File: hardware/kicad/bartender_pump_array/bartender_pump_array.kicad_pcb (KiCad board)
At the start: 2 copper layers, 56 x 61.8 mm, 43 parts, among them J1 Pump 1, J10 Pump 10, J11 12V INPUT, J12 Conn_01x12_Female, J2 Pump 2, J3 Pump 3, J4 Pump 4, J5 Pump 5, J6 Pump 6, J7 Pump 7, J8 Pump 8, J9 Pump 9, Q1 TIP120, Q10 TIP120, Q2 TIP120, Q3 TIP120, Q4 TIP120, Q5 TIP120, Q6 TIP120, Q7 TIP120, Q8 TIP120, Q9 TIP120

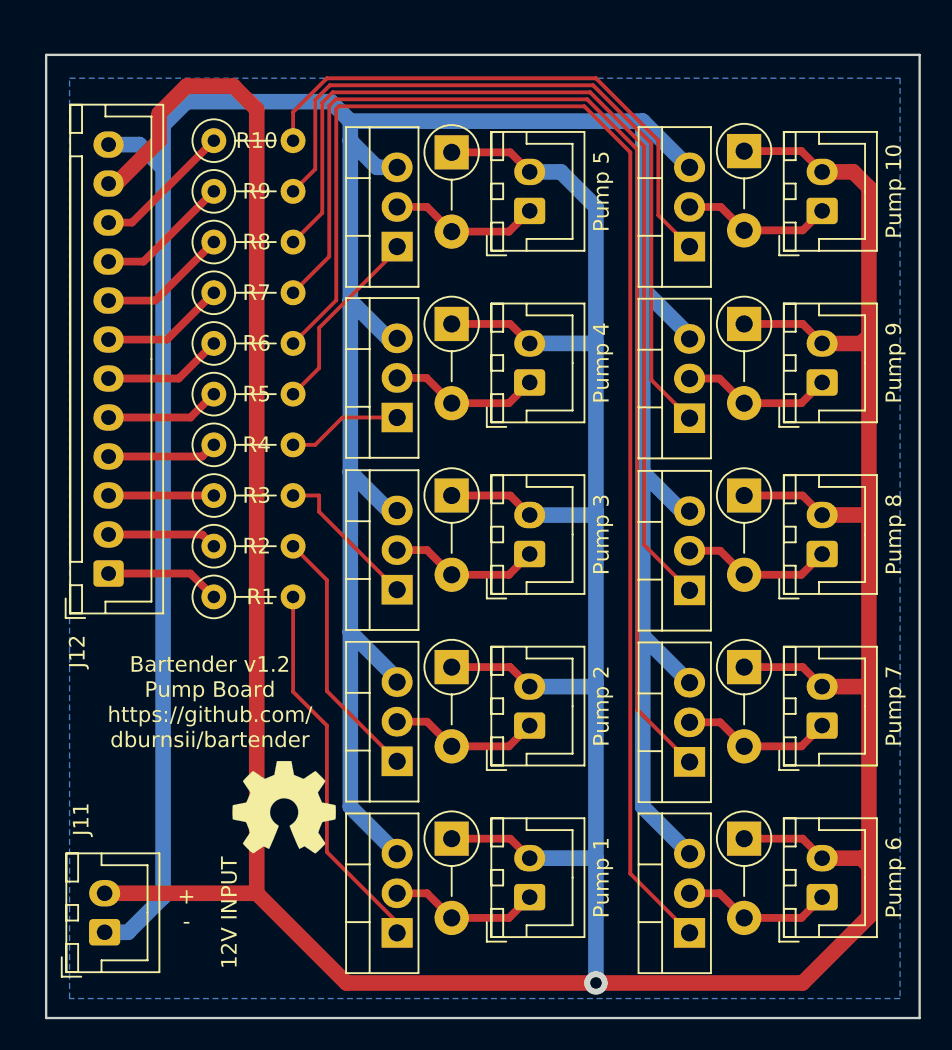
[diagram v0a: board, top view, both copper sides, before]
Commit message: Got wifi up and running, started work on the Mini
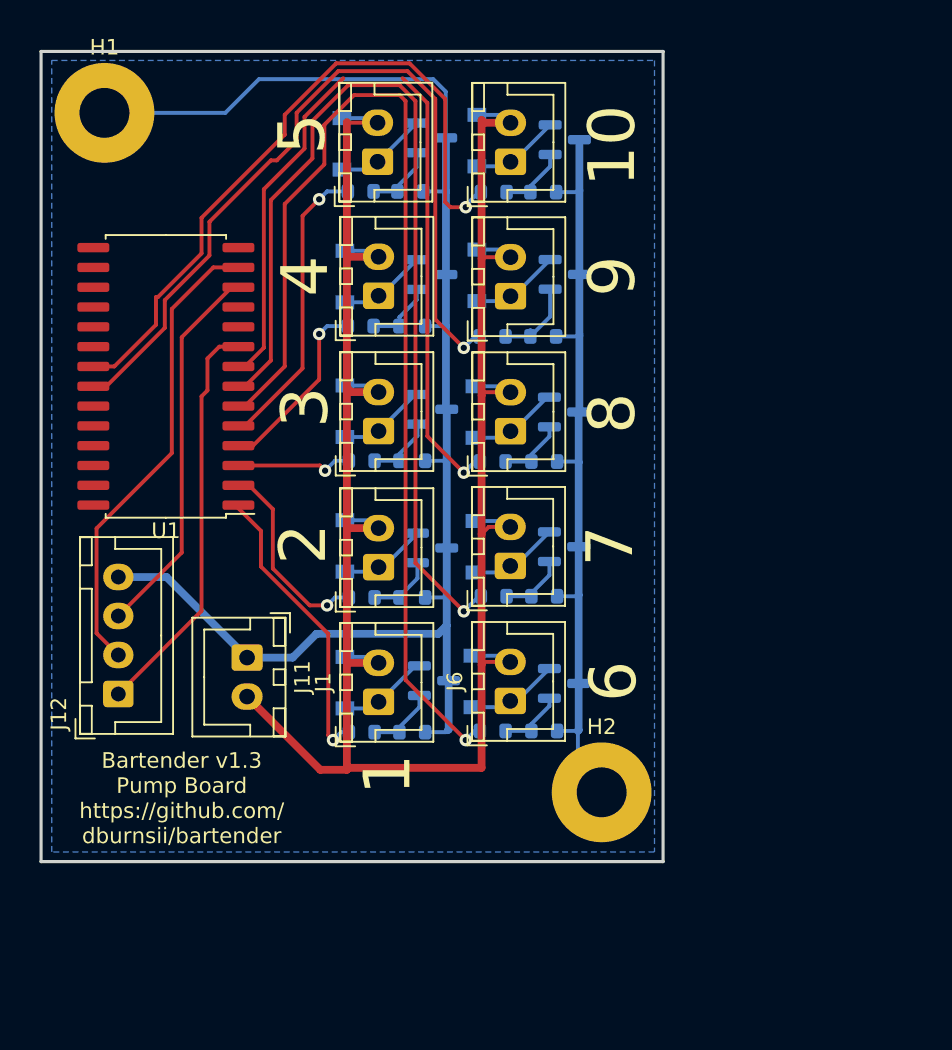
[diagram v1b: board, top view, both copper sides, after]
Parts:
- removed REF**: OSHW-Symbol_6.7x6mm_SilkScreen, Symbol:OSHW-Symbol_6.7x6mm_SilkScreen
- added H1: MountingHole_Pad, MountingHole:MountingHole_3.2mm_M3_Pad, F.Cu at (31.0, 45.5)
- added H2: MountingHole_Pad, MountingHole:MountingHole_3.2mm_M3_Pad, F.Cu at (62.9, 89.0)
- added R11: R_Small_US, Resistor_SMD:R_0603_1608Metric, B.Cu at (50.7, 85.2)
- added R12: R_Small_US, Resistor_SMD:R_0603_1608Metric, B.Cu at (50.7, 76.5)
- added R13: R_Small_US, Resistor_SMD:R_0603_1608Metric, B.Cu at (50.7, 67.8)
- added R14: R_Small_US, Resistor_SMD:R_0603_1608Metric, B.Cu at (50.7, 59.1)
- added R15: R_Small_US, Resistor_SMD:R_0603_1608Metric, B.Cu at (50.6, 50.5)
- added R16: R_Small_US, Resistor_SMD:R_0603_1608Metric, B.Cu at (59.2, 85.1)
- added R17: R_Small_US, Resistor_SMD:R_0603_1608Metric, B.Cu at (59.2, 76.5)
- added R18: R_Small_US, Resistor_SMD:R_0603_1608Metric, B.Cu at (59.2, 67.8)
- added R19: R_Small_US, Resistor_SMD:R_0603_1608Metric, B.Cu at (59.1, 59.8)
- added R20: R_Small_US, Resistor_SMD:R_0603_1608Metric, B.Cu at (59.1, 50.5)
- added U1: MCP23017_SO, Package_SO:SOIC-28W_7.5x17.9mm_P1.27mm, F.Cu at (34.9, 62.4)
- D1, D10, D2, D3, D4, D5, D6, D7, D8, D9: value DIODE -> 1N4148W; footprint Diode_THT:D_DO-41_SOD81_P5.08mm_Vertical_AnodeUp -> Diode_SMD:D_SOD-123; moved to B.Cu
- J1: value Pump 1 -> 1
- J10: value Pump 10 -> 10
- J11: value 12V INPUT -> 12V
- J12: value Conn_01x12_Female -> Conn_01x04_Female; footprint Connector_JST:JST_XH_B12B-XH-A_1x12_P2.50mm_Vertical -> Connector_JST:JST_XH_B4B-XH-A_1x04_P2.50mm_Vertical
- J2: value Pump 2 -> 2
- J3: value Pump 3 -> 3
- J4: value Pump 4 -> 4
- J5: value Pump 5 -> 5
- J6: value Pump 6 -> 6
- J7: value Pump 7 -> 7
- J8: value Pump 8 -> 8
- J9: value Pump 9 -> 9
- Q1, Q10, Q2, Q3, Q4, Q5, Q6, Q7, Q8, Q9: value TIP120 -> AO3400A; footprint Package_TO_SOT_THT:TO-220-3_Vertical -> Package_TO_SOT_SMD:SOT-23; moved to B.Cu
- R1, R10, R2, R3, R4, R5, R6, R7, R8, R9: footprint Resistor_THT:R_Axial_DIN0207_L6.3mm_D2.5mm_P5.08mm_Vertical -> Resistor_SMD:R_0603_1608Metric; moved to B.Cu
- moved R6 30.6 mm to (55.9, 85.1)
- moved R7 26.5 mm to (55.9, 76.5)
- moved J6 23.6 mm to (57.0, 83.2)
- moved R8 22.8 mm to (55.9, 67.8)
- moved J7 22.5 mm to (57.0, 74.5)
- moved J8 21.5 mm to (57.0, 65.9)
- moved J9 20.7 mm to (57.0, 57.2)
- moved J10 20.2 mm to (57.0, 48.6)
- moved R9 20.2 mm to (55.9, 59.8)
- moved D6 20.1 mm to (54.6, 81.9)
- moved J11 19.8 mm to (40.1, 80.4), turned to -90 degrees
- moved D7 18.9 mm to (54.7, 73.3)
- moved R10 18.2 mm to (55.9, 50.5)
- moved D8 18.1 mm to (54.7, 64.6)
- moved Q6 17.9 mm to (60.5, 82.0), turned to 0 degrees
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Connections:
- J12 pad 1: /P1 -> Net-(J12-Pad1)
- J12 pad 2: /P2 -> Net-(J12-Pad2)
- J12 pad 3: /P3 -> Net-(J12-Pad3)
- J12 pad 4: /P4 -> GND
- R1 pad 1: /P1 -> Net-(R1-Pad1)
- R10 pad 1: /P10 -> Net-(R10-Pad1)
- R2 pad 1: /P2 -> Net-(R2-Pad1)
- R3 pad 1: /P3 -> Net-(R3-Pad1)
- R4 pad 1: /P4 -> Net-(R4-Pad1)
- R5 pad 1: /P5 -> Net-(R5-Pad1)
- R6 pad 1: /P6 -> Net-(R6-Pad1)
- R7 pad 1: /P7 -> Net-(R7-Pad1)
- R8 pad 1: /P8 -> Net-(R8-Pad1)
- R9 pad 1: /P9 -> Net-(R9-Pad1)
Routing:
- net /12v: track 306.7 -> 144.7 mm, vias 1 -> 0
- net Net-(R6-Pad2): track 88.0 -> 4.23 mm
- net GND: track 219.7 -> 145.1 mm
- net Net-(R7-Pad2): track 74.9 -> 4.29 mm
- net Net-(R6-Pad1): track 0.00 -> 70.4 mm, vias 0 -> 1
- net Net-(R7-Pad1): track 0.00 -> 62.7 mm, vias 0 -> 1
- net Net-(R8-Pad2): track 61.7 -> 4.36 mm
- net Net-(R9-Pad1): track 0.00 -> 52.4 mm, vias 0 -> 1
- net Net-(R8-Pad1): track 0.00 -> 49.8 mm, vias 0 -> 1
- net Net-(R10-Pad1): track 0.00 -> 44.2 mm, vias 0 -> 1
- net Net-(Q9-Pad1): track 48.6 -> 5.56 mm
- net Net-(Q10-Pad1): track 35.4 -> 4.46 mm
- net Net-(J12-Pad2): track 0.00 -> 30.1 mm
- net Net-(J12-Pad1): track 0.00 -> 26.2 mm
- net Net-(J12-Pad3): track 0.00 -> 24.5 mm
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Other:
- board size 56 x 61.8 mm -> 39.9 x 51.9 mm
- net class Default removed
- board text added: "Bartender v1.3 Pump Board https://github.com/ dburnsii/bartender"
- board text removed: "+ -"
- board text removed: "Bartender v1.2 Pump Board https://github.com/ dburnsii/bartender"

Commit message: Updates for build, scale setup, new copy of pump board, etc
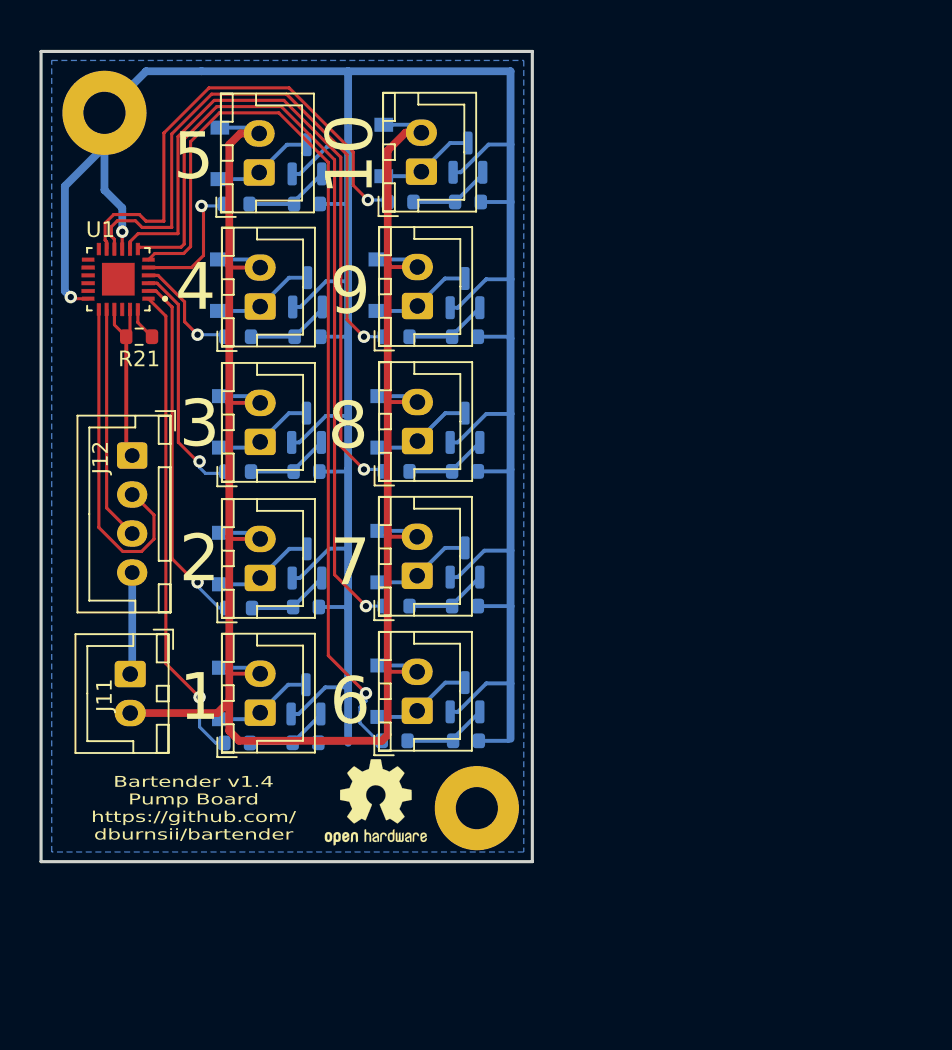
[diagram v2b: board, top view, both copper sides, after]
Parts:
- added R21: 1KR, Resistor_SMD:R_0603_1608Metric, F.Cu at (33.2, 59.8)
- added REF**: OSHW-Logo2_7.3x6mm_SilkScreen, Symbol:OSHW-Logo2_7.3x6mm_SilkScreen, F.Cu at (48.4, 89.7)
- H1, H2: footprint MountingHole:MountingHole_3.2mm_M3_Pad -> MountingHole:MountingHole_2.7mm_M2.5_Pad
- U1: value MCP23017_SO -> PCAL6416AHF,128; footprint Package_SO:SOIC-28W_7.5x17.9mm_P1.27mm -> PCAL6416AHF:QFN50P400X400X80-25N
- moved J12 15.3 mm to (32.8, 67.4), turned to -90 degrees
- moved Q1 8.30 mm to (43.9, 83.1), turned to 90 degrees
- moved Q3 8.14 mm to (43.9, 65.7), turned to 90 degrees
- moved Q2 8.08 mm to (44.0, 74.4), turned to 90 degrees
- moved Q5 8.07 mm to (44.0, 48.4), turned to 90 degrees
- moved D4 8.07 mm to (38.4, 56.5)
- moved H2 8.07 mm to (54.9, 90.0)
- moved R1 8.02 mm to (39.5, 85.9)
- moved Q4 8.02 mm to (44.0, 57.0), turned to 90 degrees
- moved R5 8.00 mm to (39.5, 51.3)
- moved D2 7.96 mm to (38.5, 74.0)
- moved D1 7.95 mm to (38.5, 82.7)
- moved R3 7.95 mm to (39.6, 68.5)
- moved D3 7.95 mm to (38.5, 65.3)
- moved R2 7.89 mm to (39.6, 77.2)
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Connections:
- D1 pad 2: Net-(J1-Pad1) -> Net-(D1-Pad2)
- D10 pad 2: Net-(J10-Pad1) -> Net-(D10-Pad2)
- D2 pad 2: Net-(J2-Pad1) -> Net-(D2-Pad2)
- D3 pad 2: Net-(J3-Pad1) -> Net-(D3-Pad2)
- D4 pad 2: Net-(J4-Pad1) -> Net-(D4-Pad2)
- D5 pad 2: Net-(J5-Pad1) -> Net-(D5-Pad2)
- D6 pad 2: Net-(J6-Pad1) -> Net-(D6-Pad2)
- D7 pad 2: Net-(J7-Pad1) -> Net-(D7-Pad2)
- D8 pad 2: Net-(J8-Pad1) -> Net-(D8-Pad2)
- D9 pad 2: Net-(J9-Pad1) -> Net-(D9-Pad2)
- J1 pad 1: Net-(J1-Pad1) -> Net-(D1-Pad2)
- J10 pad 1: Net-(J10-Pad1) -> Net-(D10-Pad2)
- J12 pad 1: Net-(J12-Pad1) -> +3V3
- J2 pad 1: Net-(J2-Pad1) -> Net-(D2-Pad2)
- J3 pad 1: Net-(J3-Pad1) -> Net-(D3-Pad2)
- J4 pad 1: Net-(J4-Pad1) -> Net-(D4-Pad2)
- J5 pad 1: Net-(J5-Pad1) -> Net-(D5-Pad2)
- J6 pad 1: Net-(J6-Pad1) -> Net-(D6-Pad2)
- J7 pad 1: Net-(J7-Pad1) -> Net-(D7-Pad2)
- J8 pad 1: Net-(J8-Pad1) -> Net-(D8-Pad2)
- J9 pad 1: Net-(J9-Pad1) -> Net-(D9-Pad2)
- Q1 pad 1: Net-(R1-Pad2) -> Net-(Q1-Pad1)
- Q1 pad 2: Net-(J1-Pad1) -> GND
- Q1 pad 3: GND -> Net-(D1-Pad2)
- Q10 pad 2: Net-(J10-Pad1) -> GND
- Q10 pad 3: GND -> Net-(D10-Pad2)
- Q2 pad 1: Net-(R2-Pad2) -> Net-(Q2-Pad1)
- Q2 pad 2: Net-(J2-Pad1) -> GND
- Q2 pad 3: GND -> Net-(D2-Pad2)
- Q3 pad 1: Net-(R3-Pad2) -> Net-(Q3-Pad1)
- Q3 pad 2: Net-(J3-Pad1) -> GND
- Q3 pad 3: GND -> Net-(D3-Pad2)
- Q4 pad 1: Net-(R4-Pad2) -> Net-(Q4-Pad1)
- Q4 pad 2: Net-(J4-Pad1) -> GND
- Q4 pad 3: GND -> Net-(D4-Pad2)
- Q5 pad 1: Net-(R5-Pad2) -> Net-(Q5-Pad1)
- Q5 pad 2: Net-(J5-Pad1) -> GND
- Q5 pad 3: GND -> Net-(D5-Pad2)
- Q6 pad 1: Net-(R6-Pad2) -> Net-(Q6-Pad1)
- Q6 pad 2: Net-(J6-Pad1) -> GND
- Q6 pad 3: GND -> Net-(D6-Pad2)
- Q7 pad 1: Net-(R7-Pad2) -> Net-(Q7-Pad1)
- Q7 pad 2: Net-(J7-Pad1) -> GND
- Q7 pad 3: GND -> Net-(D7-Pad2)
- Q8 pad 1: Net-(R8-Pad2) -> Net-(Q8-Pad1)
- Q8 pad 2: Net-(J8-Pad1) -> GND
- Q8 pad 3: GND -> Net-(D8-Pad2)
- Q9 pad 2: Net-(J9-Pad1) -> GND
- Q9 pad 3: GND -> Net-(D9-Pad2)
- R1 pad 2: Net-(R1-Pad2) -> Net-(Q1-Pad1)
- R11 pad 1: GND -> Net-(Q1-Pad1)
- R11 pad 2: Net-(R1-Pad2) -> GND
- R12 pad 1: GND -> Net-(Q2-Pad1)
- R12 pad 2: Net-(R2-Pad2) -> GND
- R13 pad 1: GND -> Net-(Q3-Pad1)
- R13 pad 2: Net-(R3-Pad2) -> GND
- R14 pad 1: GND -> Net-(Q4-Pad1)
- R14 pad 2: Net-(R4-Pad2) -> GND
- R15 pad 1: GND -> Net-(Q5-Pad1)
- R15 pad 2: Net-(R5-Pad2) -> GND
- R16 pad 1: GND -> Net-(Q6-Pad1)
- R16 pad 2: Net-(R6-Pad2) -> GND
- R17 pad 1: GND -> Net-(Q7-Pad1)
- R17 pad 2: Net-(R7-Pad2) -> GND
- R18 pad 1: GND -> Net-(Q8-Pad1)
- R18 pad 2: Net-(R8-Pad2) -> GND
- R19 pad 1: GND -> Net-(Q9-Pad1)
- R19 pad 2: Net-(Q9-Pad1) -> GND
- R2 pad 2: Net-(R2-Pad2) -> Net-(Q2-Pad1)
- R20 pad 1: GND -> Net-(Q10-Pad1)
- R20 pad 2: Net-(Q10-Pad1) -> GND
- R3 pad 2: Net-(R3-Pad2) -> Net-(Q3-Pad1)
- R4 pad 2: Net-(R4-Pad2) -> Net-(Q4-Pad1)
- R5 pad 2: Net-(R5-Pad2) -> Net-(Q5-Pad1)
- R6 pad 2: Net-(R6-Pad2) -> Net-(Q6-Pad1)
- R7 pad 2: Net-(R7-Pad2) -> Net-(Q7-Pad1)
- R8 pad 2: Net-(R8-Pad2) -> Net-(Q8-Pad1)
- U1 pad 10: unconnected-(U1-Pad10) -> Net-(R9-Pad1)
- U1 pad 11: unconnected-(U1-Pad11) -> Net-(R10-Pad1)
- U1 pad 12: Net-(J12-Pad3) -> unconnected-(U1-Pad12)
- U1 pad 13: Net-(J12-Pad2) -> unconnected-(U1-Pad13)
- U1 pad 18: unconnected-(U1-Pad18) -> GND
- U1 pad 19: unconnected-(U1-Pad19) -> Net-(J12-Pad2)
- U1 pad 20: unconnected-(U1-Pad20) -> Net-(J12-Pad3)
- U1 pad 21: Net-(R10-Pad1) -> +3V3
- U1 pad 22: Net-(R9-Pad1) -> unconnected-(U1-Pad22)
- U1 pad 23: unconnected-(U1-Pad23) -> +3V3
- U1 pad 24: unconnected-(U1-Pad24) -> Net-(R21-Pad1)
- U1 pad 9: Net-(J12-Pad1) -> GND
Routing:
- net GND: track 145.1 -> 207.1 mm, vias 0 -> 2
- net Net-(J12-Pad1): track 26.2 -> 0.00 mm
- net Net-(R9-Pad1): track 52.4 -> 39.0 mm
- net Net-(R10-Pad1): track 44.2 -> 31.4 mm
- net Net-(R1-Pad1): track 18.8 -> 30.8 mm
- net +3V3: track 0.00 -> 11.7 mm
- net Net-(R6-Pad1): track 70.4 -> 59.2 mm
- net Net-(R5-Pad1): track 19.0 -> 8.55 mm
- net Net-(R7-Pad1): track 62.7 -> 52.3 mm
- net Net-(R2-Pad1): track 12.7 -> 22.6 mm
- net Net-(J12-Pad3): track 24.5 -> 15.0 mm
- net Net-(J12-Pad2): track 30.1 -> 22.0 mm
- net Net-(R3-Pad1): track 7.48 -> 15.4 mm
- net Net-(J5-Pad1): track 6.88 -> 0.00 mm
- net Net-(D4-Pad2): track 0.00 -> 6.54 mm
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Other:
- board size 39.9 x 51.9 mm -> 31.5 x 51.9 mm
- board text added: "Bartender v1.4 Pump Board https://github.com/ dburnsii/bartender"
- board text removed: "Bartender v1.3 Pump Board https://github.com/ dburnsii/bartender"
